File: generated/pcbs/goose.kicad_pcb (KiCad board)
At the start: 2 copper layers, 131.7 x 96.3 mm, 65 parts

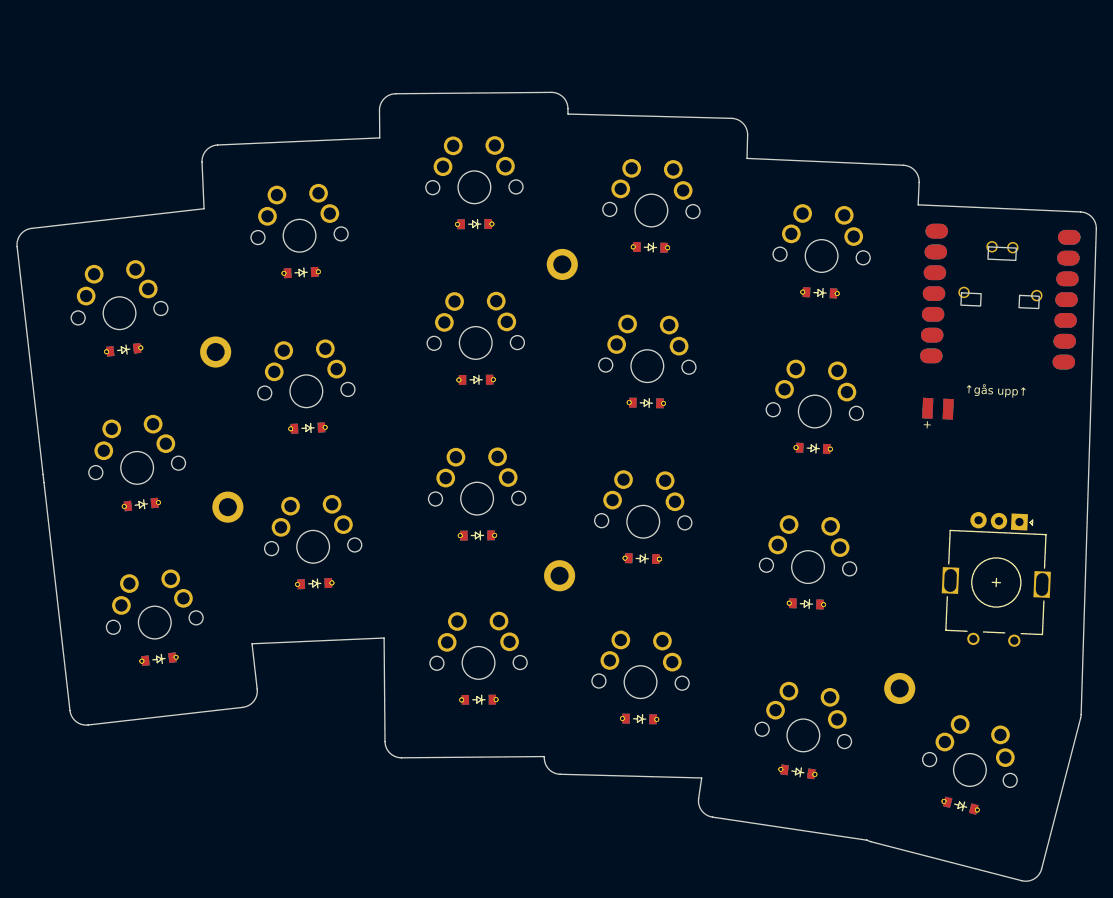
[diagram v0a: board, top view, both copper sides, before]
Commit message: Start messing around with choc
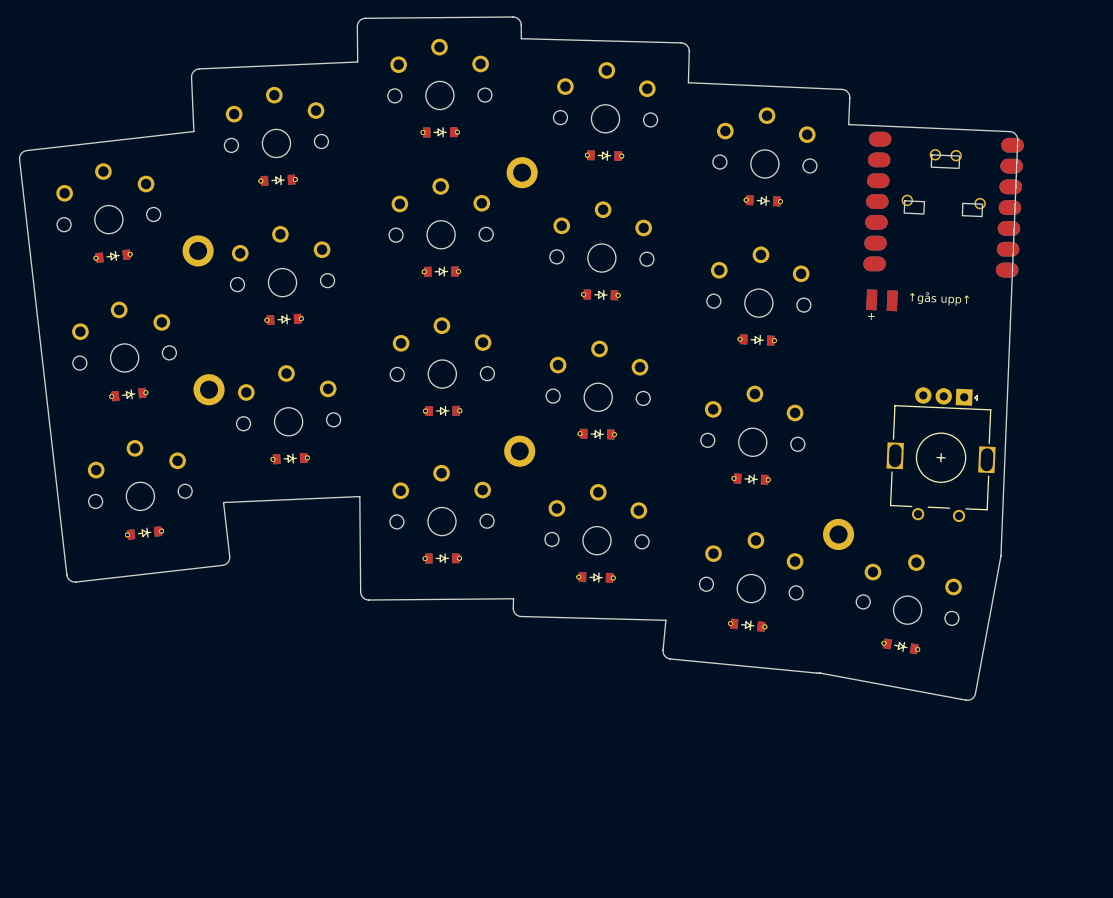
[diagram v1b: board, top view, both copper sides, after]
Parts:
- S1, S10, S11, S12, S13, S14, S15, S16, S17, S18, S19, S2, S3, S4, S5, S6, S7, S8, S9: footprint MX -> PG1350
- moved S19 20.9 mm to (271.7, 163.7), turned to -10.5 degrees
- moved Di19 20.8 mm to (270.9, 168.1), turned to 169.5 degrees
- moved Di38 20.8 mm to (270.9, 168.1), turned to 169.5 degrees
- moved H5 20.2 mm to (263.3, 154.4), turned to -8 degrees
- moved S18 19.0 mm to (252.7, 161.1), turned to -5.5 degrees
- moved Di18 18.9 mm to (252.2, 165.5), turned to 174.5 degrees
- moved Di37 18.9 mm to (252.2, 165.5), turned to 174.5 degrees
- moved Di17 18.1 mm to (233.7, 159.7)
- moved Di36 18.1 mm to (233.7, 159.7)
- moved S17 18.1 mm to (233.8, 155.2)
- moved Di16 17.8 mm to (214.9, 157.4)
- moved Di35 17.8 mm to (214.9, 157.4)
- moved S16 17.8 mm to (214.9, 152.9)
- moved Di13 16.7 mm to (252.6, 147.7)
- moved Di32 16.7 mm to (252.6, 147.7)
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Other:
- board size 131.7 x 96.3 mm -> 121.8 x 83.4 mm
